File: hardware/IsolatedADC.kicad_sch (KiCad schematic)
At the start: 21 parts, among them IC3 OPA1679-Q1, IC4 ADS131M04, IC5 LTC1799

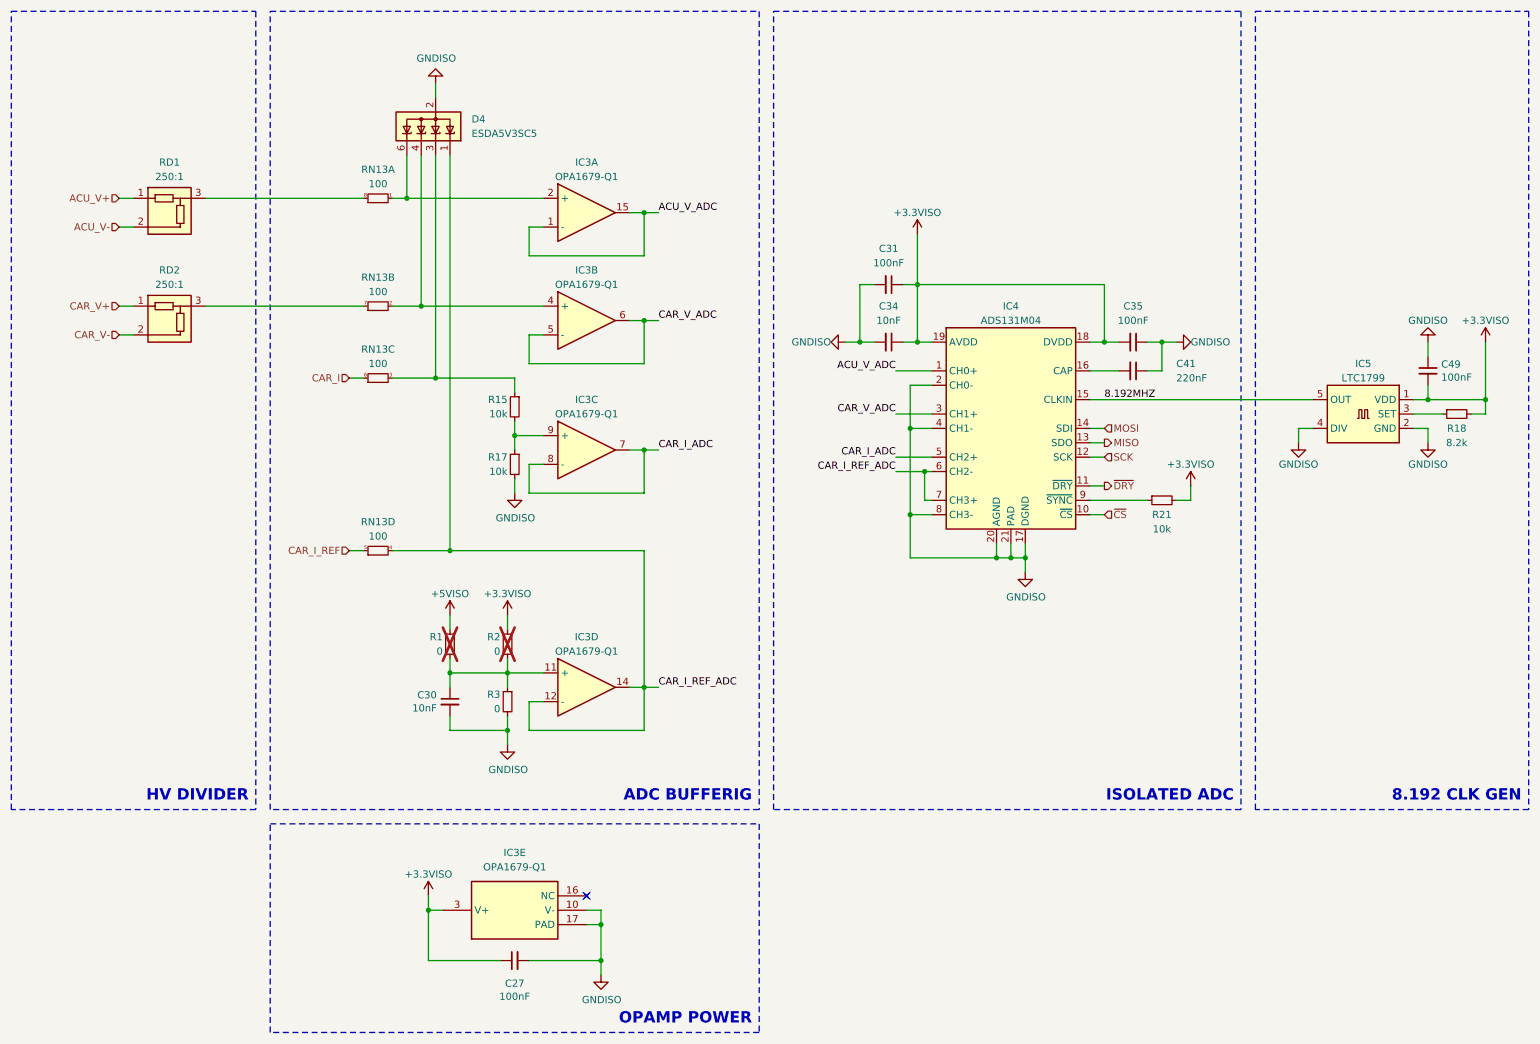
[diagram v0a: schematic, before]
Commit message: mama comit
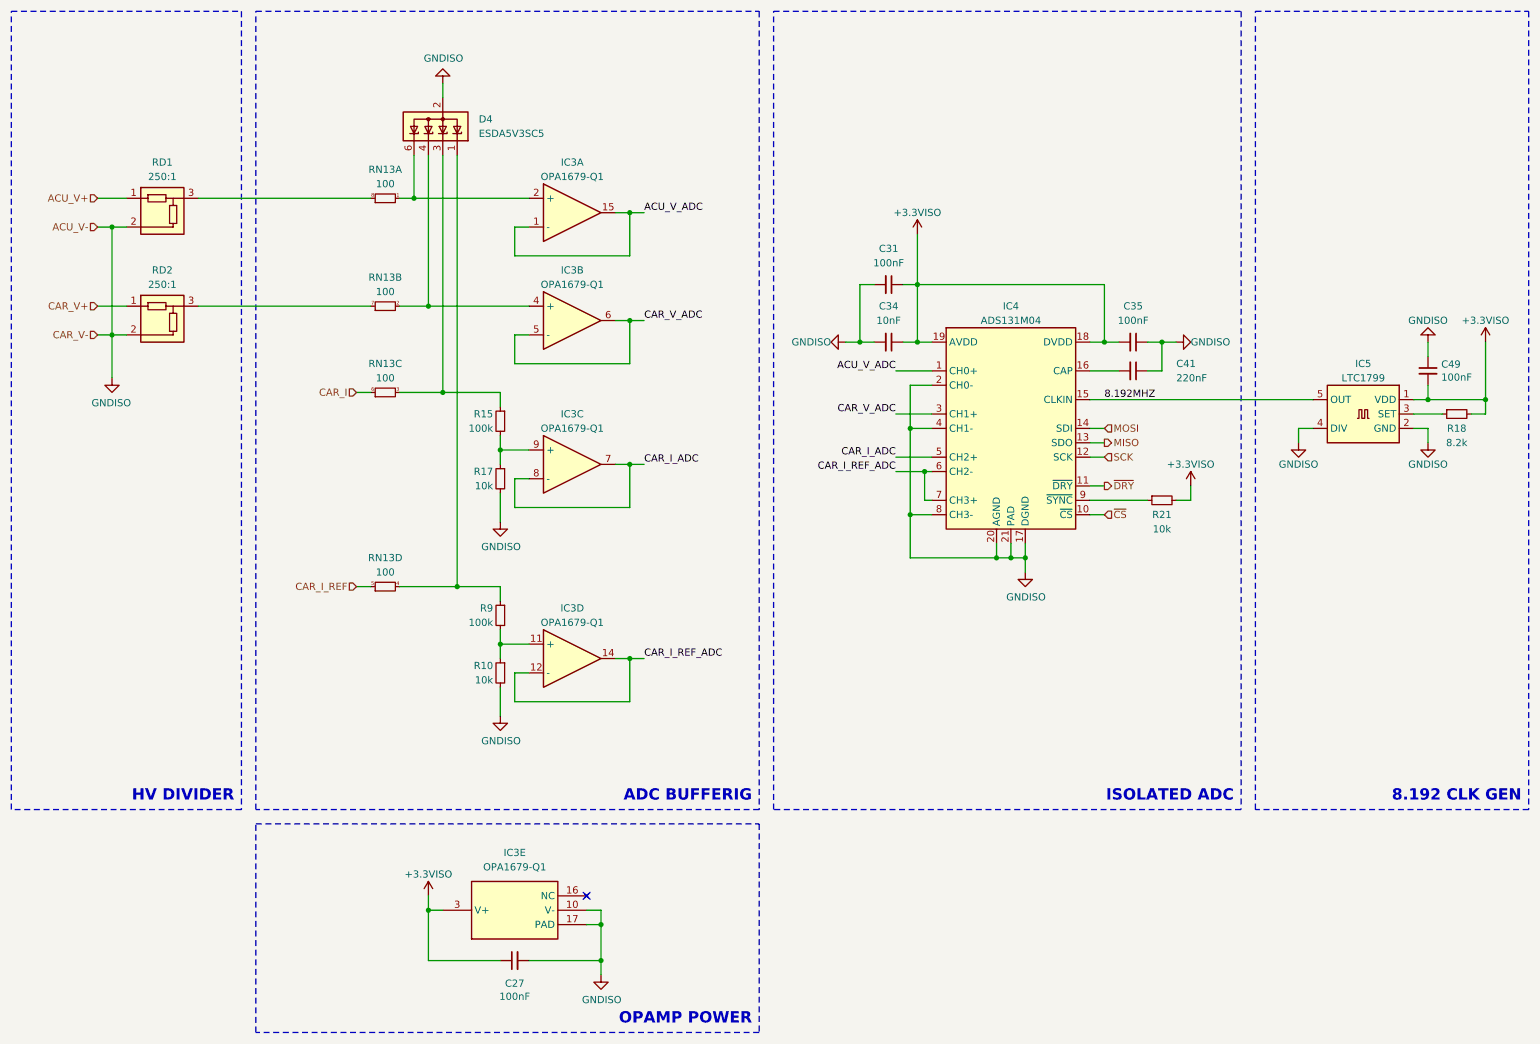
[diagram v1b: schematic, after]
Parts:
- removed C30: 10nF, Capacitor_SMD:C_0603_1608Metric, symbol Device:C_Small
- removed R1, R2, R3: 0, Resistor_SMD:R_0603_1608Metric, symbol Device:R_Small
- added R10: 10k, Resistor_SMD:R_0603_1608Metric, symbol Device:R_Small
- added R9: 100k, Resistor_SMD:R_0603_1608Metric, symbol Device:R_Small
- R15: value 10k -> 100k
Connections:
- net ACU_V- is gone; now on net GNDISO: RD1.2
- net CAR_V- is gone; now on net GNDISO: RD2.2
- net CAR_I_REF_ADC: no longer D4.1 (A), RN13.4 (R4.1)
- net GNDISO: now also R10.2
- net at IC3.11 (+): now also R10.1, R9.2
- new net: D4.1 (A), R9.1, RN13.4 (R4.1)
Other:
- moved on the sheet: D4, IC3A, IC3B, IC3C, IC3D, R15, R17, RD1, RD2, RN13A, RN13B, RN13C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
